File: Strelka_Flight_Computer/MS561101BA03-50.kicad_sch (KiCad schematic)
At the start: 2 parts, among them U12 MS561101BA03-50

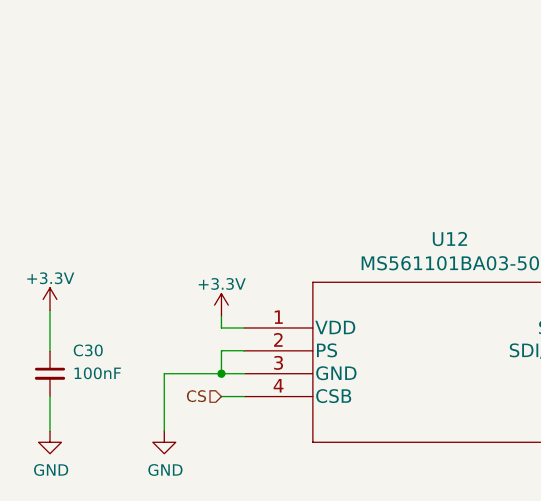
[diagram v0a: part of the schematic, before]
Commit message: Continued routing
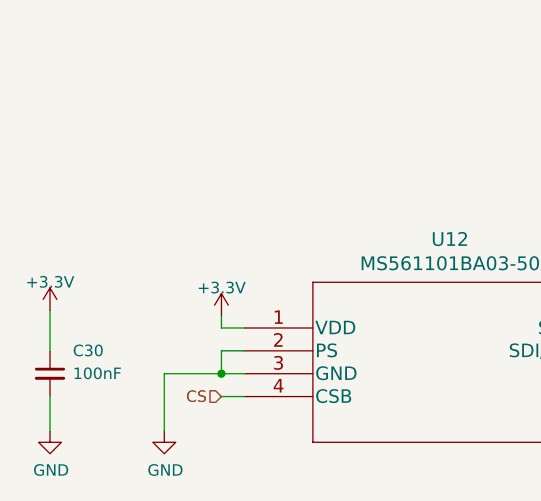
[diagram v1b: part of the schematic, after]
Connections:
- net +3V3 renamed +3.3V
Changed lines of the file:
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@@
+    )
+  )
+  (symbol (lib_name "+3.3V_1") (lib_id "power:+3.3V") (at 104.775 87.63 0) (unit 1)
+    (in_bom yes) (on_board yes) (dnp no) (fields_autoplaced)
+    (property "Reference" "#PWR07" (at 104.775 91.44 0)
+      (effects (font (size 1.27 1.27)) hide)
+    )
+    (property "Value" "+3.3V" (at 104.775 84.455 0)
+      (effects (font (size 1.27 1.27)))
+    )
+    (property "Footprint" "" (at 104.775 87.63 0)
+      (effects (font (size 1.27 1.27)) hide)
+    )
+    (property "Datasheet" "" (at 104.775 87.63 0)
+      (effects (font (size 1.27 1.27)) hide)
+    )
+    (pin "1")
+    (instances
+      (project "Strelka_Flight_Computer"
+        (path "/e63e39d7-6ac0-4ffd-8aa3-1841a4541b55/e94c6cea-6c6c-4b5f-a840-b97a15d9406a"
+          (reference "#PWR07") (unit 1)
+        )
+        (path "/e63e39d7-6ac0-4ffd-8aa3-1841a4541b55/78f71895-bddb-4f64-a608-99074f2d1c44/9f95701d-2876-4223-990f-d706d5845c81"
+          (reference "#PWR010") (unit 1)
+        )
+      )
     )
   )
@@
     )
   )
-  (symbol (lib_id "power:+3.3V") (at 104.775 87.63 0) (unit 1)
+  (symbol (lib_name "+3.3V_1") (lib_id "power:+3.3V") (at 123.825 88.265 0) (unit 1)
     (in_bom yes) (on_board yes) (dnp no) (fields_autoplaced)
-    (property "Reference" "#PWR0178" (at 104.775 91.44 0)
+    (property "Reference" "#PWR07" (at 123.825 92.075 0)
       (effects (font (size 1.27 1.27)) hide)
     )
-    (property "Value" "+3.3V" (at 104.775 84.0542 0)
+    (property "Value" "+3.3V" (at 123.825 85.09 0)
       (effects (font (size 1.27 1.27)))
     )
-    (property "Footprint" "" (at 104.775 87.63 0)
+    (property "Footprint" "" (at 123.825 88.265 0)
       (effects (font (size 1.27 1.27)) hide)
     )
-    (property "Datasheet" "" (at 104.775 87.63 0)
+    (property "Datasheet" "" (at 123.825 88.265 0)
       (effects (font (size 1.27 1.27)) hide)
     )
@@
     (instances
       (project "Strelka_Flight_Computer"
+        (path "/e63e39d7-6ac0-4ffd-8aa3-1841a4541b55/e94c6cea-6c6c-4b5f-a840-b97a15d9406a"
+          (reference "#PWR07") (unit 1)
+        )
         (path "/e63e39d7-6ac0-4ffd-8aa3-1841a4541b55/78f71895-bddb-4f64-a608-99074f2d1c44/9f95701d-2876-4223-990f-d706d5845c81"
-          (reference "#PWR0178") (unit 1)
+          (reference "#PWR03") (unit 1)
         )
       )
@@
         )
       )
-    )
-  )
-  (symbol (lib_id "power:+3.3V") (at 123.825 88.265 0) (unit 1)
-    (in_bom yes) (on_board yes) (dnp no) (fields_autoplaced)
-    (property "Reference" "#PWR0181" (at 123.825 92.075 0)
-      (effects (font (size 1.27 1.27)) hide)
-    )
-    (property "Value" "+3.3V" (at 123.825 84.6892 0)
-      (effects (font (size 1.27 1.27)))
-    )
-    (property "Footprint" "" (at 123.825 88.265 0)
-      (effects (font (size 1.27 1.27)) hide)
-    )
-    (property "Datasheet" "" (at 123.825 88.265 0)
-      (effects (font (size 1.27 1.27)) hide)
-    )
-    (pin "1")
-    (instances
-      (project "Strelka_Flight_Computer"
-        (path "/e63e39d7-6ac0-4ffd-8aa3-1841a4541b55/78f71895-bddb-4f64-a608-99074f2d1c44/9f95701d-2876-4223-990f-d706d5845c81"
-          (reference "#PWR0181") (unit 1)
-        )
-      )
